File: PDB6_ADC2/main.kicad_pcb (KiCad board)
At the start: 2 copper layers, 20 x 16 mm, 27 parts, among them P1 CONN_01X08, P2 CONN_01X03, P3 CONN_01X03, P4 CONN_01X08, U1 ADS7828

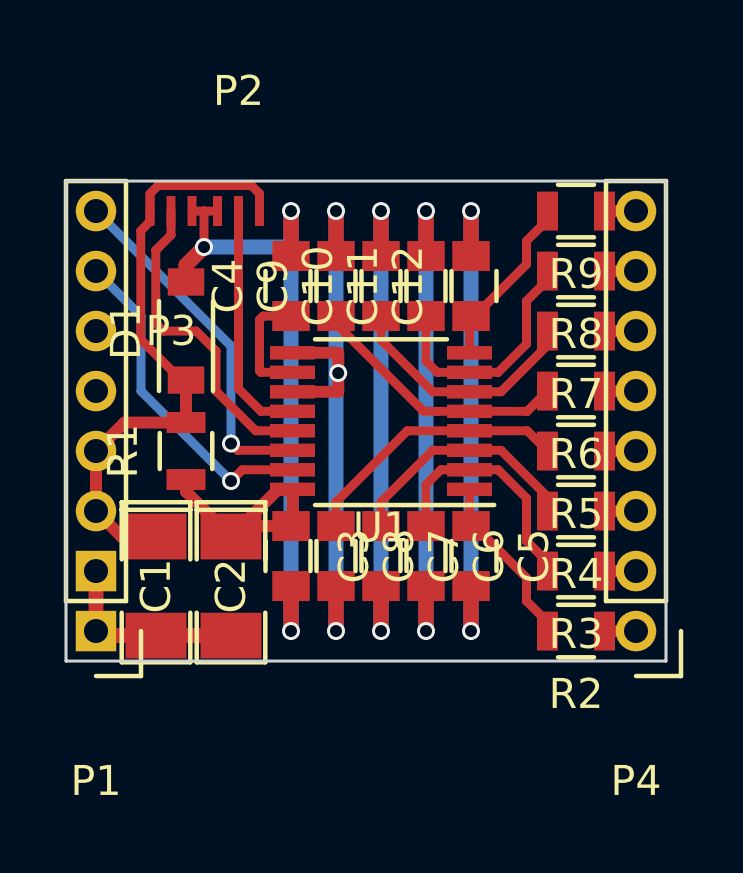
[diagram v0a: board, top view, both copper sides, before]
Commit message: test
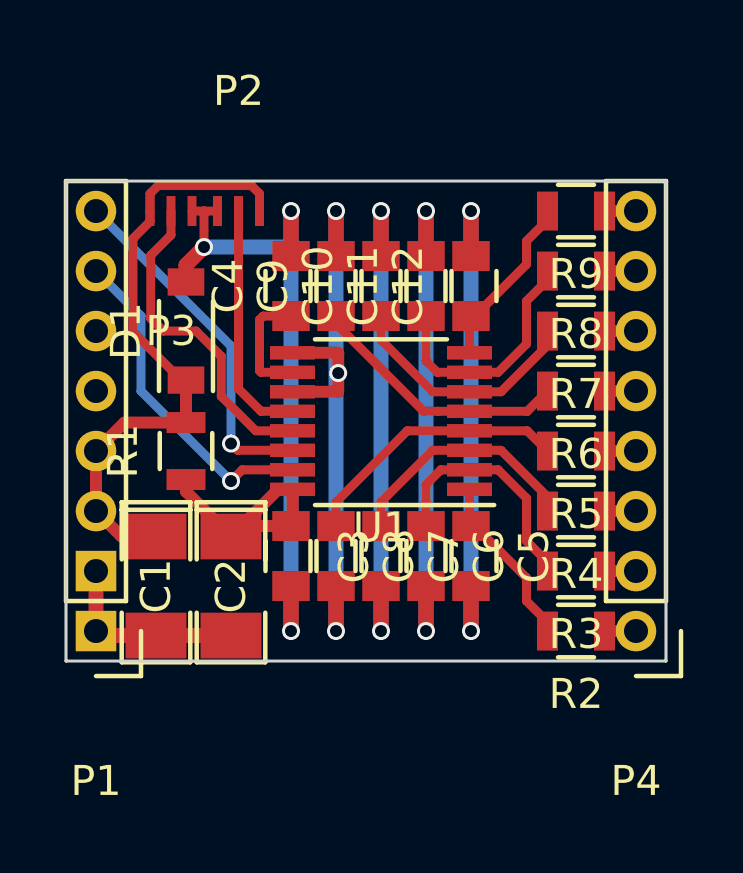
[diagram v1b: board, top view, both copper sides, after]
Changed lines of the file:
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@@
-(kicad_pcb (version 4) (host pcbnew 4.0.4-stable)
+(kicad_pcb (version 4) (host pcbnew 4.0.4+e1-6308~48~ubuntu16.04.1-stable)
   (general
     (links 56)
@@
   )
   (setup
-    (last_trace_width 0.3)
+    (last_trace_width 0.25)
     (user_trace_width 0.3)
     (user_trace_width 0.4)
@@
   (gr_line (start 185 141) (end 185 125) (layer Edge.Cuts) (width 0.1))
   (segment (start 187.8 126) (end 187.8 126.35) (width 0.3) (layer F.Cu) (net 1))
-  (segment (start 187.8 126.35) (end 187.493481 126.656519) (width 0.3) (layer F.Cu) (net 1))
-  (segment (start 187.493481 130.283481) (end 188.845 131.635) (width 0.3) (layer F.Cu) (net 1))
-  (segment (start 187.493481 126.656519) (end 187.493481 130.283481) (width 0.3) (layer F.Cu) (net 1))
+  (segment (start 187.8 126.35) (end 187.233535 126.916465) (width 0.3) (layer F.Cu) (net 1))
+  (segment (start 187.233535 126.916465) (end 187.233535 130.023535) (width 0.3) (layer F.Cu) (net 1))
   (segment (start 188.845 131.635) (end 189 131.635) (width 0.3) (layer F.Cu) (net 1))
+  (segment (start 187.233535 130.023535) (end 188.845 131.635) (width 0.3) (layer F.Cu) (net 1))
   (segment (start 189 131.635) (end 189 133.05) (width 0.4) (layer F.Cu) (net 1))
   (segment (start 189 133.05) (end 186.95 133.05) (width 0.4) (layer F.Cu) (net 1))
@@
   (segment (start 191.5 132.675) (end 192.55 132.675) (width 0.3) (layer F.Cu) (net 15))
   (segment (start 188.5 126) (end 188.5 126.8) (width 0.3) (layer F.Cu) (net 16))
-  (segment (start 188.5 126.8) (end 187.993491 127.306509) (width 0.3) (layer F.Cu) (net 16))
-  (segment (start 187.993491 127.306509) (end 187.993491 129.745634) (width 0.3) (layer F.Cu) (net 16))
-  (segment (start 187.993491 129.745634) (end 188.247857 130) (width 0.3) (layer F.Cu) (net 16))
+  (segment (start 187.824522 127.475478) (end 187.824522 129.576665) (width 0.3) (layer F.Cu) (net 16))
+  (segment (start 188.5 126.8) (end 187.824522 127.475478) (width 0.3) (layer F.Cu) (net 16))
+  (segment (start 187.824522 129.576665) (end 188.247857 130) (width 0.3) (layer F.Cu) (net 16))
   (segment (start 188.247857 130) (end 189.335369 130) (width 0.3) (layer F.Cu) (net 16))
-  (segment (start 189.335369 130) (end 190 130.664631) (width 0.3) (layer F.Cu) (net 16))
-  (segment (start 190 130.664631) (end 190 132) (width 0.3) (layer F.Cu) (net 16))
   (segment (start 191.325 133.325) (end 192.55 133.325) (width 0.3) (layer F.Cu) (net 16))
-  (segment (start 190 132) (end 191.325 133.325) (width 0.3) (layer F.Cu) (net 16))
+  (segment (start 189.335369 130) (end 190.175338 130.839969) (width 0.3) (layer F.Cu) (net 16))
+  (segment (start 190.175338 130.839969) (end 190.175338 132.175338) (width 0.3) (layer F.Cu) (net 16))
+  (segment (start 190.175338 132.175338) (end 191.325 133.325) (width 0.3) (layer F.Cu) (net 16))
   (segment (start 202.95 140) (end 204 140) (width 0.4) (layer F.Cu) (net 17))
   (segment (start 204 138) (end 202.95 138) (width 0.4) (layer F.Cu) (net 18))
